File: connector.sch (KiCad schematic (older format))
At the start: 2 parts, among them J301 SEAM-50-02.0-S-08-2-A-K-TR-ND, J302 SEAF-50-05.0-S-08-2-A-K-TR

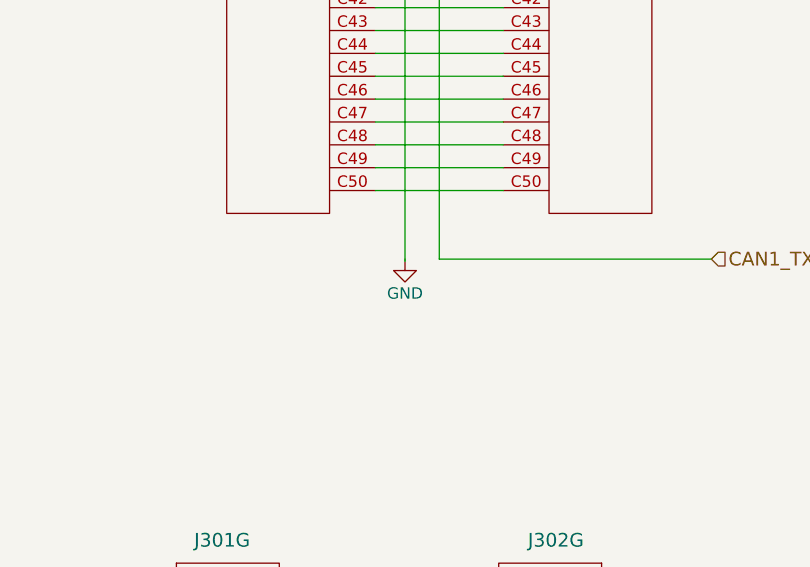
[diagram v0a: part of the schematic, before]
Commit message: Finish layout and generate Gerber files
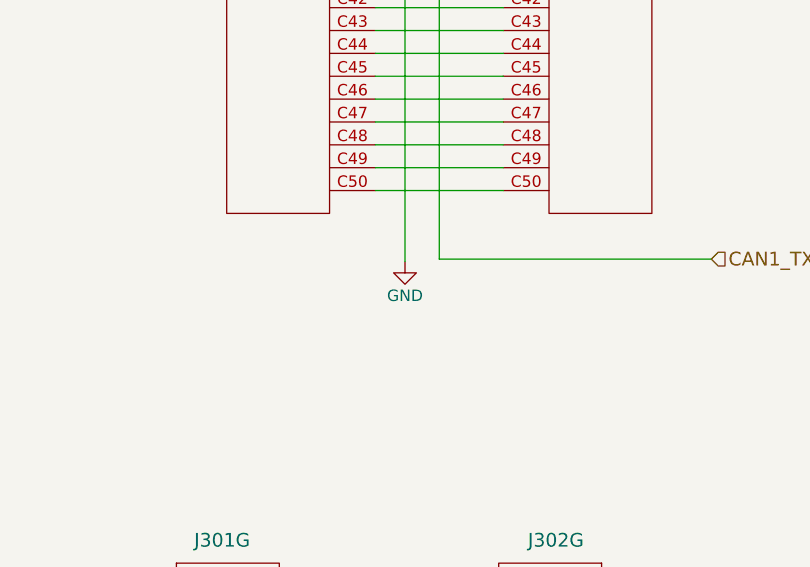
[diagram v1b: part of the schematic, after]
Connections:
- net GND: now also J301.C3, J301.C4, J302.C3, J302.C4
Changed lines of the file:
@@
 L GND #PWR018
 U 1 1 5A56619A
-P 11920 6560
-F 0 "#PWR018" H 11920 6310 50  0001 C CNN
-F 1 "GND" H 11920 6410 50  0000 C CNN
-F 2 "" H 11920 6560 50  0001 C CNN
-F 3 "" H 11920 6560 50  0001 C CNN
-	1    11920 6560
+P 11920 6570
+F 0 "#PWR018" H 11920 6320 50  0001 C CNN
+F 1 "GND" H 11920 6420 50  0000 C CNN
+F 2 "" H 11920 6570 50  0001 C CNN
+F 3 "" H 11920 6570 50  0001 C CNN
+	1    11920 6570
 	1    0    0    -1
 $EndComp
